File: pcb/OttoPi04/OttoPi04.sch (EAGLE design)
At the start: 26 parts

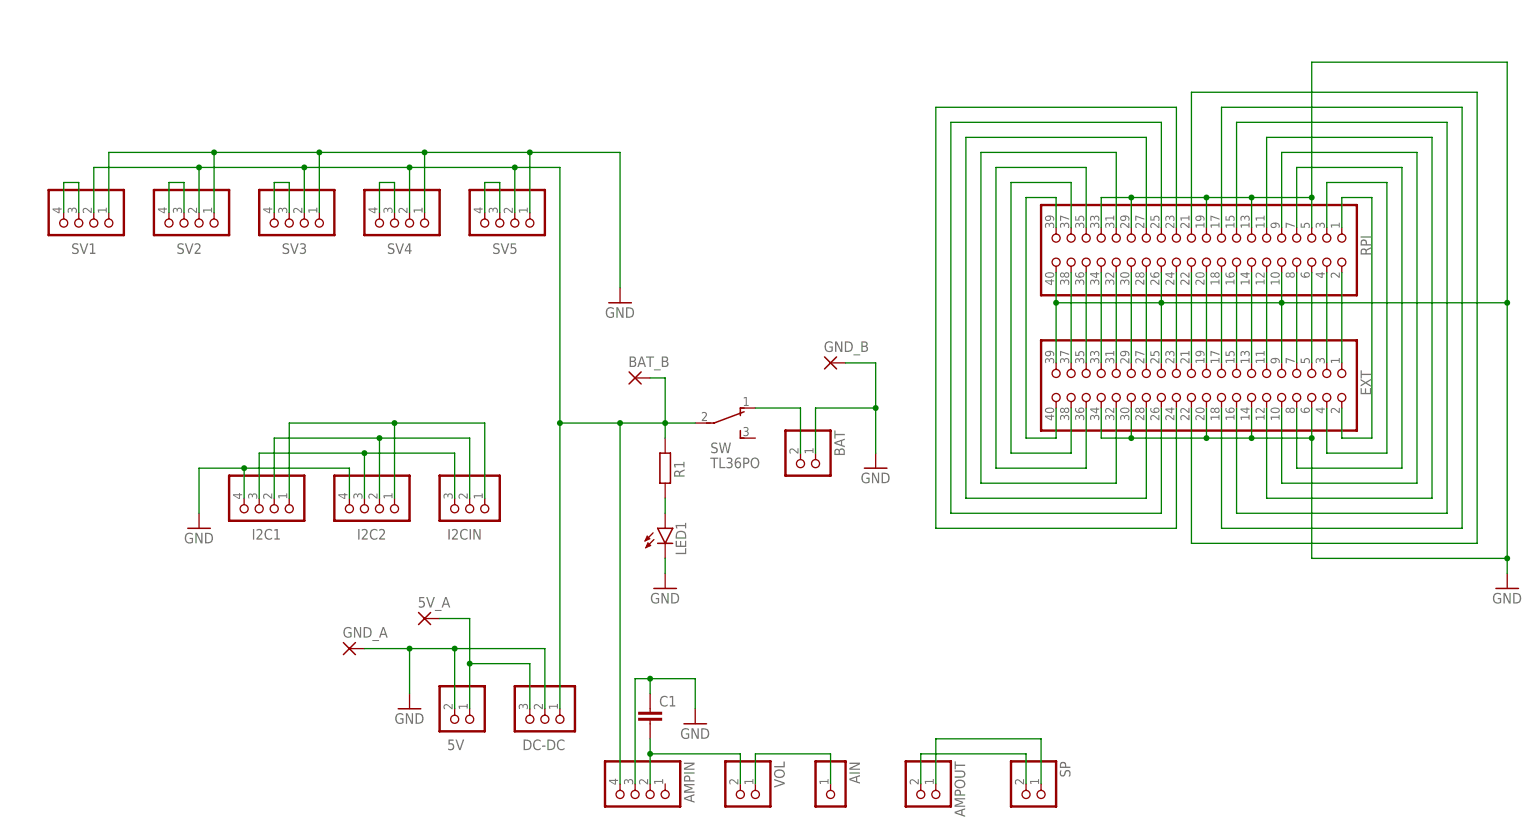
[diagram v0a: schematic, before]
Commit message: pcb
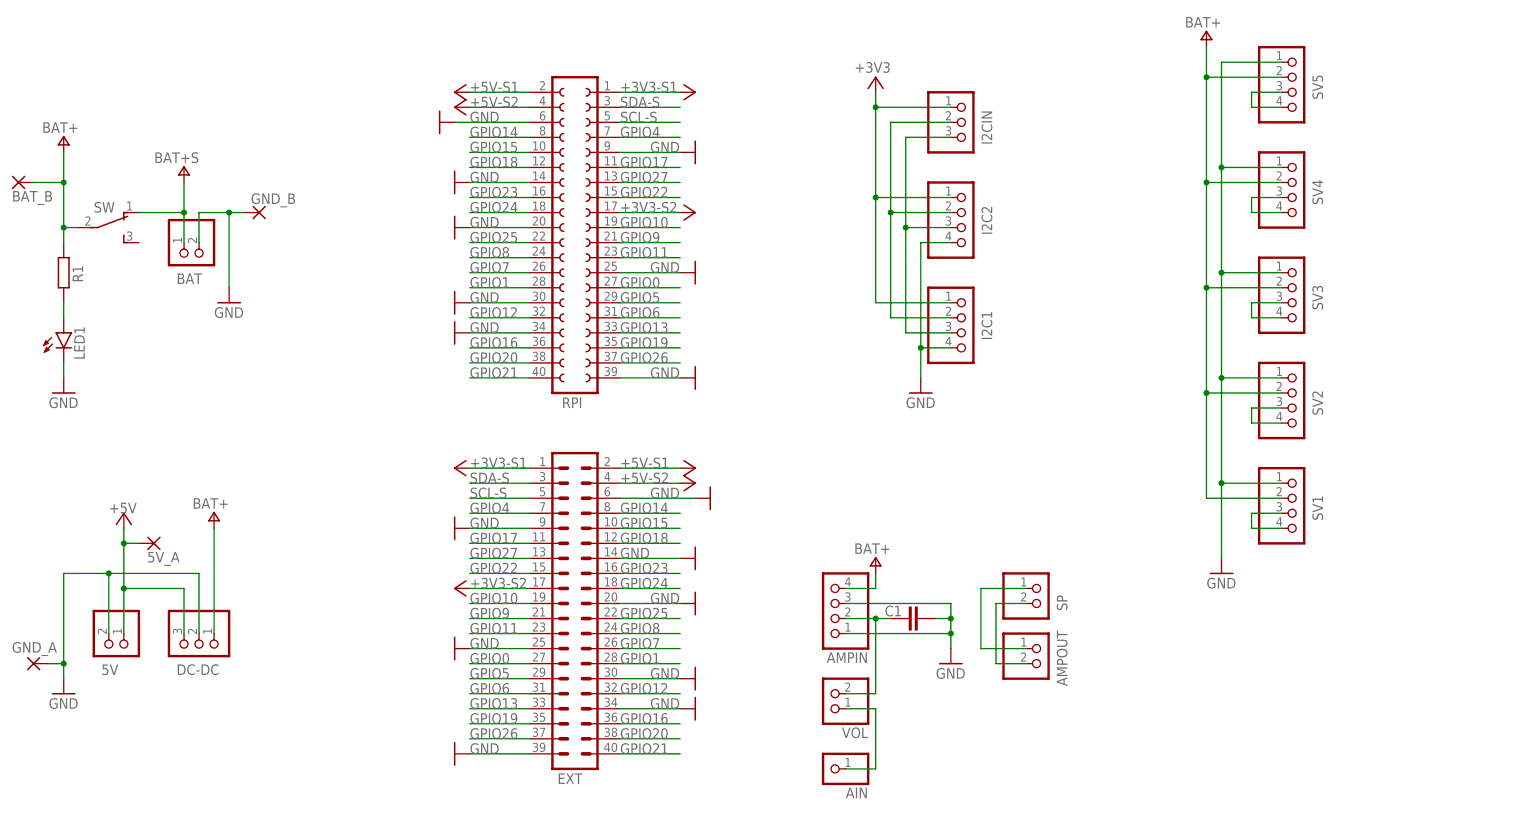
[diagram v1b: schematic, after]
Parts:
- BAT: device pinhead:PINHD-1X2 -> adafruit:JST_2PIN-THM
- EXT: device pinhead:PINHD-2X20 -> con-lstb:MA20-2W
- RPI: device pinhead:PINHD-2X20 -> con-lsta:FE20-2
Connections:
- net 3V3 renamed +3V3
- net 5V renamed +5V
- removed net 3V: EXT.1, RPI.2
- removed net 4V: AMPIN.4, BAT_B.P, DC-DC.1, R1.2, SV1.2, SV2.2, SV3.2, SV4.2, SV5.2, SW.P
- removed net 5V1: EXT.2, RPI.1
- removed net 5V2: EXT.4, RPI.3
- removed net N$1: EXT.28, RPI.27
- removed net N$10: EXT.7, RPI.8
- removed net N$12: EXT.11, RPI.12
- removed net N$13: EXT.13, RPI.14
- removed net N$14: EXT.15, RPI.16
- removed net N$17: EXT.19, RPI.20
- removed net N$18: EXT.21, RPI.22
- removed net N$19: EXT.23, RPI.24
- removed net N$2: EXT.17, RPI.18
- removed net N$21: EXT.27, RPI.28
- removed net N$22: EXT.29, RPI.30
- removed net N$23: EXT.31, RPI.32
- removed net N$24: EXT.33, RPI.34
- removed net N$25: EXT.35, RPI.36
- removed net N$26: EXT.37, RPI.38
- removed net N$28: EXT.12, RPI.11
- removed net N$30: EXT.16, RPI.15
- removed net N$31: EXT.40, RPI.39
- removed net N$32: EXT.38, RPI.37
- removed net N$35: EXT.32, RPI.31
- removed net N$38: EXT.26, RPI.25
- removed net N$39: EXT.24, RPI.23
- removed net N$4: EXT.3, RPI.4
- removed net N$41: EXT.18, RPI.17
- removed net N$43: EXT.10, RPI.9
- removed net N$5: EXT.5, RPI.6
- removed net N$6: EXT.22, RPI.21
- removed net N$7: EXT.36, RPI.35
- removed net N$9: EXT.8, RPI.7
- new net +3V3-S1: EXT.1, RPI.1
- new net +3V3-S2: EXT.17, RPI.17
- new net +4V_S: BAT.2, SW.O
- new net +5V-S1: EXT.2, RPI.2
- new net +5V-S2: EXT.4, RPI.4
- new net GPIO0: EXT.27, RPI.27
- new net GPIO1: EXT.28, RPI.28
- new net GPIO10: EXT.19, RPI.19
- new net GPIO11: EXT.23, RPI.23
- new net GPIO12: EXT.32, RPI.32
- new net GPIO13: EXT.33, RPI.33
- new net GPIO14: EXT.8, RPI.8
- new net GPIO15: EXT.10, RPI.10
- new net GPIO16: EXT.36, RPI.36
- new net GPIO17: EXT.11, RPI.11
- new net GPIO18: EXT.12, RPI.12
- new net GPIO19: EXT.35, RPI.35
- new net GPIO20: EXT.38, RPI.38
- new net GPIO21: EXT.40, RPI.40
- new net GPIO22: EXT.15, RPI.15
- new net GPIO23: EXT.16, RPI.16
- new net GPIO24: EXT.18, RPI.18
- new net GPIO25: EXT.22, RPI.22
- new net GPIO26: EXT.37, RPI.37
- new net GPIO27: EXT.13, RPI.13
- new net GPIO4: EXT.7, RPI.7
- new net GPIO5: EXT.29, RPI.29
- new net GPIO6: EXT.31, RPI.31
- new net GPIO7: EXT.26, RPI.26
- new net GPIO8: EXT.24, RPI.24
- new net GPIO9: EXT.21, RPI.21
- new net SCL-S: EXT.5, RPI.5
- new net SDA-S: EXT.3, RPI.3
- net BAT+: now also AMPIN.4, BAT_B.P, DC-DC.1, R1.2, SV1.2, SV2.2, SV3.2, SV4.2, SV5.2, SW.P; no longer BAT.2, SW.O
- net GND: now also AMPIN.1, RPI.14, RPI.20, RPI.25, RPI.30, RPI.34, RPI.39, RPI.6, RPI.9; no longer RPI.10, RPI.13, RPI.19, RPI.26, RPI.29, RPI.33, RPI.40, RPI.5
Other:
- moved on the sheet: 5V, 5V_A, AIN, AMPIN, AMPOUT, BAT, BAT_B, C1, DC-DC, GND_A, GND_B, I2C1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
